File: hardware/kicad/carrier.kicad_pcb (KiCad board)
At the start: 2 copper layers, 105 x 95 mm, 116 parts, among them J1 MC-107DMS, J10 J_ADS_MAIN ADSBee J5, J11 J_ADS_GNSS ADSBee J4, J2 J_NTC 103AT-2, J3 J_BAT JST-PH 2mm, J4 J_THERM 60C NC, J5 J_GNSS GPS-18037 J5, J6 J_ESP_A support, J7 J_ESP_B power/UART, J8 J_ESP_C I2C, J9 J_ESP_D support, Q1 2N7002, Q2 2N7002, Q3 2N7002, Q4 2N7002, Q5 MMBT3904, SW1 POWER JS102011SAQN (2=common), SW2 MUTE JS102011SAQN (2=common), U1 TPS70933DBVR, U10 BMP581, U2 TUSB320LAIRWBR, U3 SN74LVC1G02DBVR, U4 BQ25606RGER, U5 TLV840CADL29DBVR 2.9V, U6 TPS61088RHLR, U7 TPS22975DSGR, U8 MAX17048G+T10, U9 SN74LVC1G17DBVR

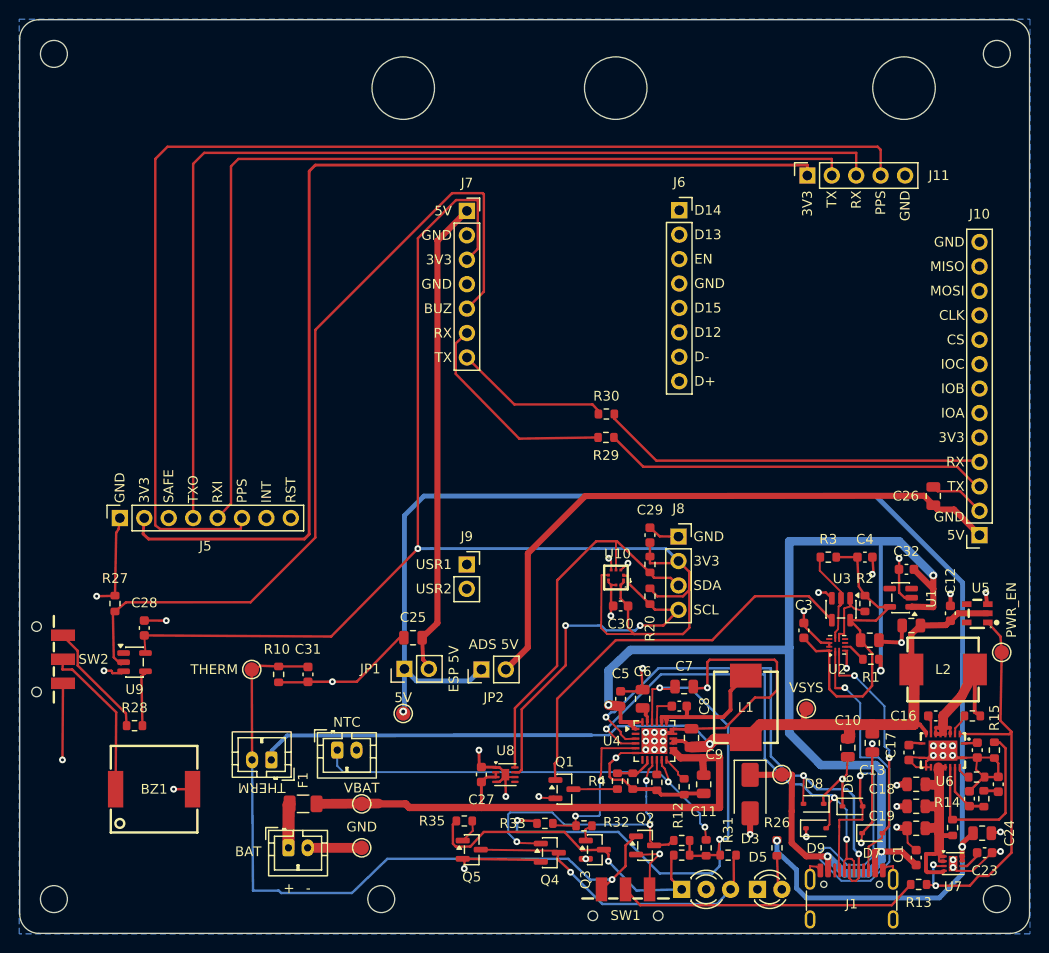
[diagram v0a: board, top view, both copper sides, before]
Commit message: Routing
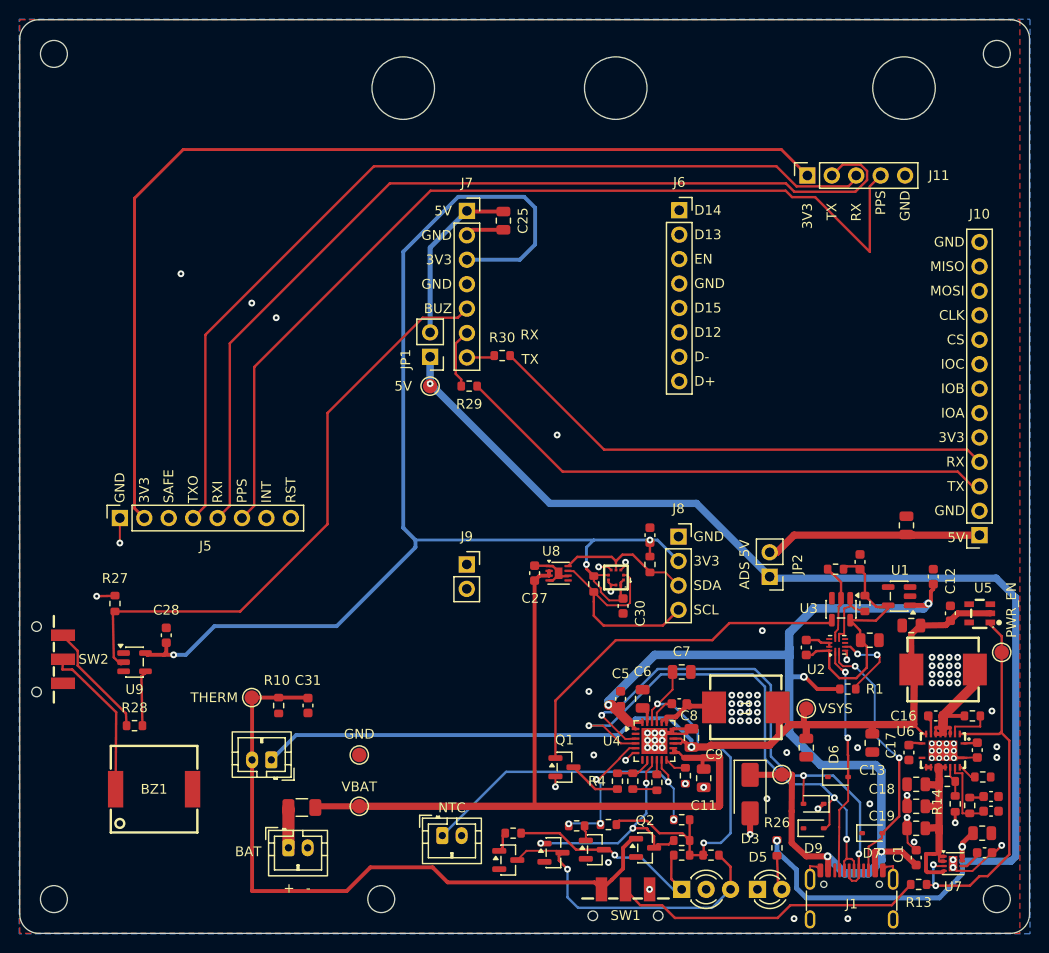
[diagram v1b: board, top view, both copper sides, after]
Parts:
- SW2: footprint SW-SMD_JS102011SAQN -> carrier:SW-SMD_JS102011SAQN
- moved C25 44.4 mm to (50.3, 20.9), turned to -90 degrees
- moved TP7 34.2 mm to (42.7, 38.1)
- moved JP1 32.6 mm to (42.7, 35.1), turned to 180 degrees
- moved JP2 31.5 mm to (78.0, 57.9), turned to 180 degrees
- moved C27 21.7 mm to (53.5, 57.5)
- moved U8 21.7 mm to (56.0, 57.6)
- moved R29 15.2 mm to (46.7, 38.1)
- moved J2 14.1 mm to (43.9, 84.8)
- moved R30 12.4 mm to (50.2, 34.9)
- moved TP6 9.66 mm to (35.3, 76.5)
- moved R15 6.91 mm to (97.3, 81.5)
- moved R33 6.61 mm to (61.2, 83.7), turned to 180 degrees
- moved R20 5.98 mm to (59.7, 58.7)
- moved R35 5.24 mm to (51.3, 84.6), turned to 180 degrees
- moved R14 4.83 mm to (96.5, 79.2), turned to 0 degrees
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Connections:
- J1 pad A8: (no net) -> unconnected-(J1-SBU1-PadA8)
- J1 pad B8: (no net) -> unconnected-(J1-SBU2-PadB8)
- J10 pad 10: (no net) -> unconnected-(J10-Pin_10-Pad10)
- J10 pad 11: (no net) -> unconnected-(J10-Pin_11-Pad11)
- J10 pad 12: (no net) -> unconnected-(J10-Pin_12-Pad12)
- J10 pad 5: (no net) -> unconnected-(J10-Pin_5-Pad5)
- J10 pad 6: (no net) -> unconnected-(J10-Pin_6-Pad6)
- J10 pad 7: (no net) -> unconnected-(J10-Pin_7-Pad7)
- J10 pad 8: (no net) -> unconnected-(J10-Pin_8-Pad8)
- J10 pad 9: (no net) -> unconnected-(J10-Pin_9-Pad9)
- J5 pad 3: (no net) -> unconnected-(J5-Pin_3-Pad3)
- J5 pad 7: (no net) -> unconnected-(J5-Pin_7-Pad7)
- J5 pad 8: (no net) -> unconnected-(J5-Pin_8-Pad8)
- J6 pad 1: (no net) -> unconnected-(J6-Pin_1-Pad1)
- J6 pad 2: (no net) -> unconnected-(J6-Pin_2-Pad2)
- J6 pad 3: (no net) -> unconnected-(J6-Pin_3-Pad3)
- J6 pad 5: (no net) -> unconnected-(J6-Pin_5-Pad5)
- J6 pad 6: (no net) -> unconnected-(J6-Pin_6-Pad6)
- J6 pad 7: (no net) -> unconnected-(J6-Pin_7-Pad7)
- J6 pad 8: (no net) -> unconnected-(J6-Pin_8-Pad8)
- J9 pad 1: (no net) -> unconnected-(J9-Pin_1-Pad1)
- J9 pad 2: (no net) -> unconnected-(J9-Pin_2-Pad2)
- U1 pad 3: (no net) -> unconnected-(U1-EN-Pad3)
- U1 pad 4: (no net) -> unconnected-(U1-NC-Pad4)
- U2 pad 5: (no net) -> unconnected-(U2-ADDR-Pad5)
- U2 pad 6: (no net) -> unconnected-(U2-INT_N/OUT3-Pad6)
- U2 pad 9: (no net) -> unconnected-(U2-ID-Pad9)
- U4 pad 2: (no net) -> unconnected-(U4-NC-Pad2)
- U4 pad 7: (no net) -> unconnected-(U4-~{PG}-Pad7)
- U5 pad 4: (no net) -> unconnected-(U5-NC-Pad4)
- U5 pad 5: (no net) -> unconnected-(U5-CT-Pad5)
- U8 pad 5: (no net) -> unconnected-(U8-~{ALRT}-Pad5)
- U9 pad 1: (no net) -> unconnected-(U9-NC-Pad1)
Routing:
- net GND: track 227.6 -> 57.7 mm, vias 53 -> 90
- net ADS_5V: track 65.5 -> 22.6 mm
- net USB_CC1: track 64.9 -> 23.8 mm
- net VBAT: track 61.3 -> 93.3 mm
- net ESP_5V: track 49.8 -> 17.9 mm
- net GNSS_PPS: track 127.0 -> 98.9 mm
- net I2C_SDA: track 40.5 -> 14.3 mm
- net USB_VBUS: track 141.4 -> 115.3 mm
- net BUZZ_PWM: track 88.1 -> 62.4 mm
- net REGN: track 63.4 -> 43.5 mm, vias 3 -> 2
- net ADS_COMMS_TX: track 40.1 -> 56.6 mm
- net BOOST_FB: track 19.5 -> 3.20 mm
- net ESP_UART_RX: track 22.4 -> 6.26 mm
- net RAIL_5V: track 150.7 -> 135.8 mm
- net I2C_SCL: track 38.3 -> 23.5 mm, vias 2 -> 0
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- added copper zone on F.Cu, net GND
